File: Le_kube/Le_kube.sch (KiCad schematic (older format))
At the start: 1 part

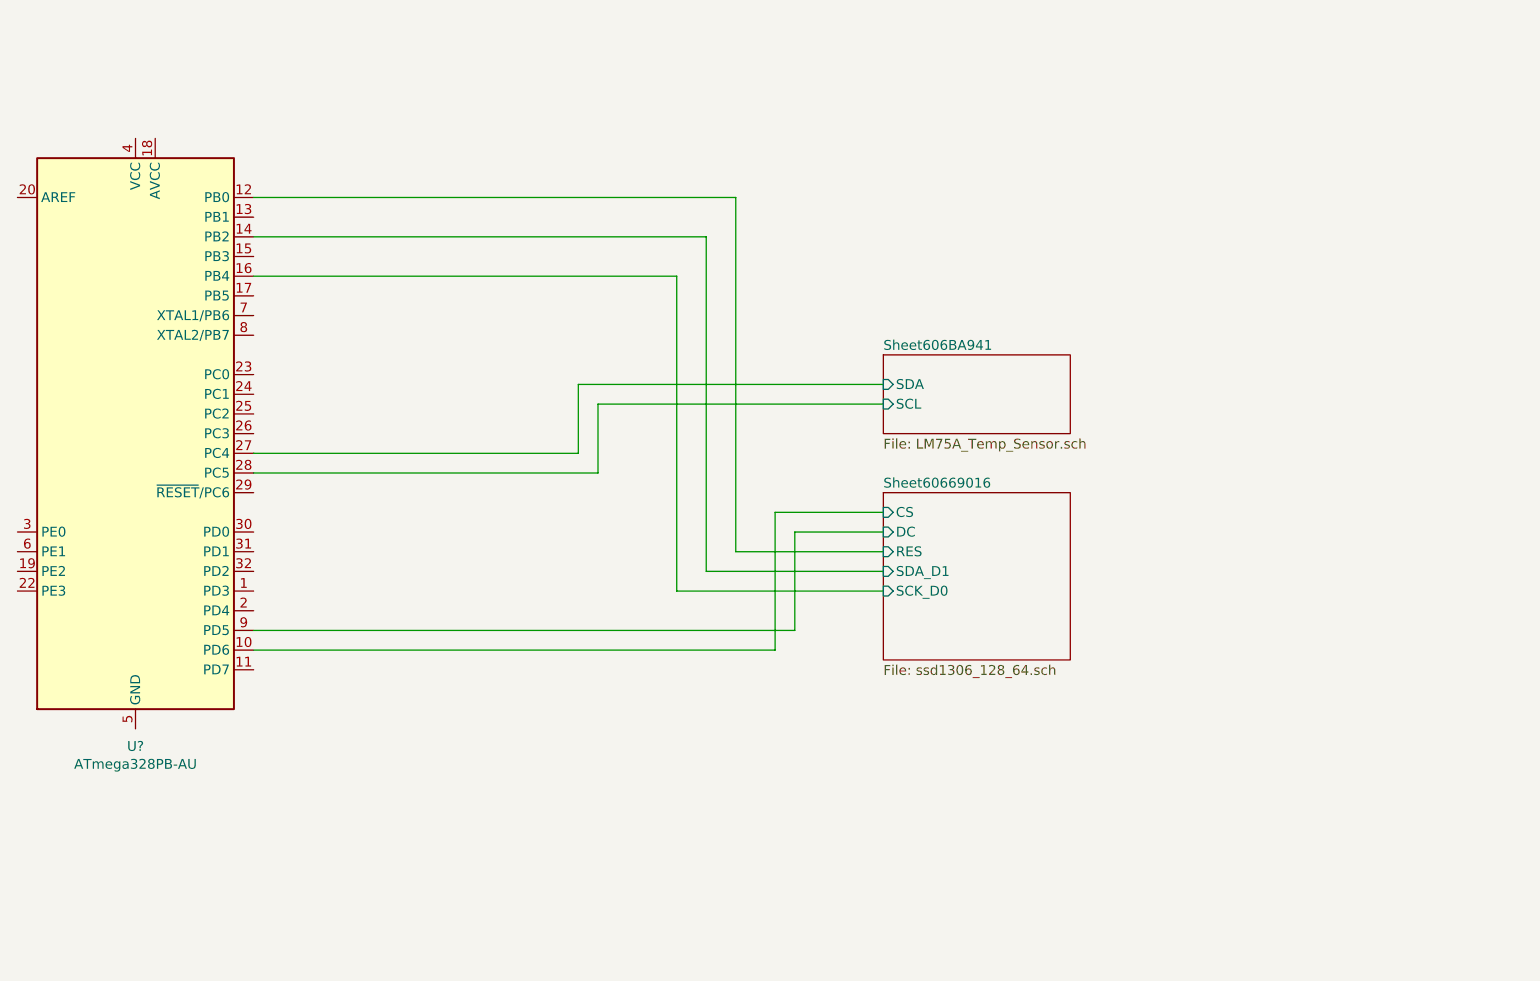
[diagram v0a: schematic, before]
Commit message: cao
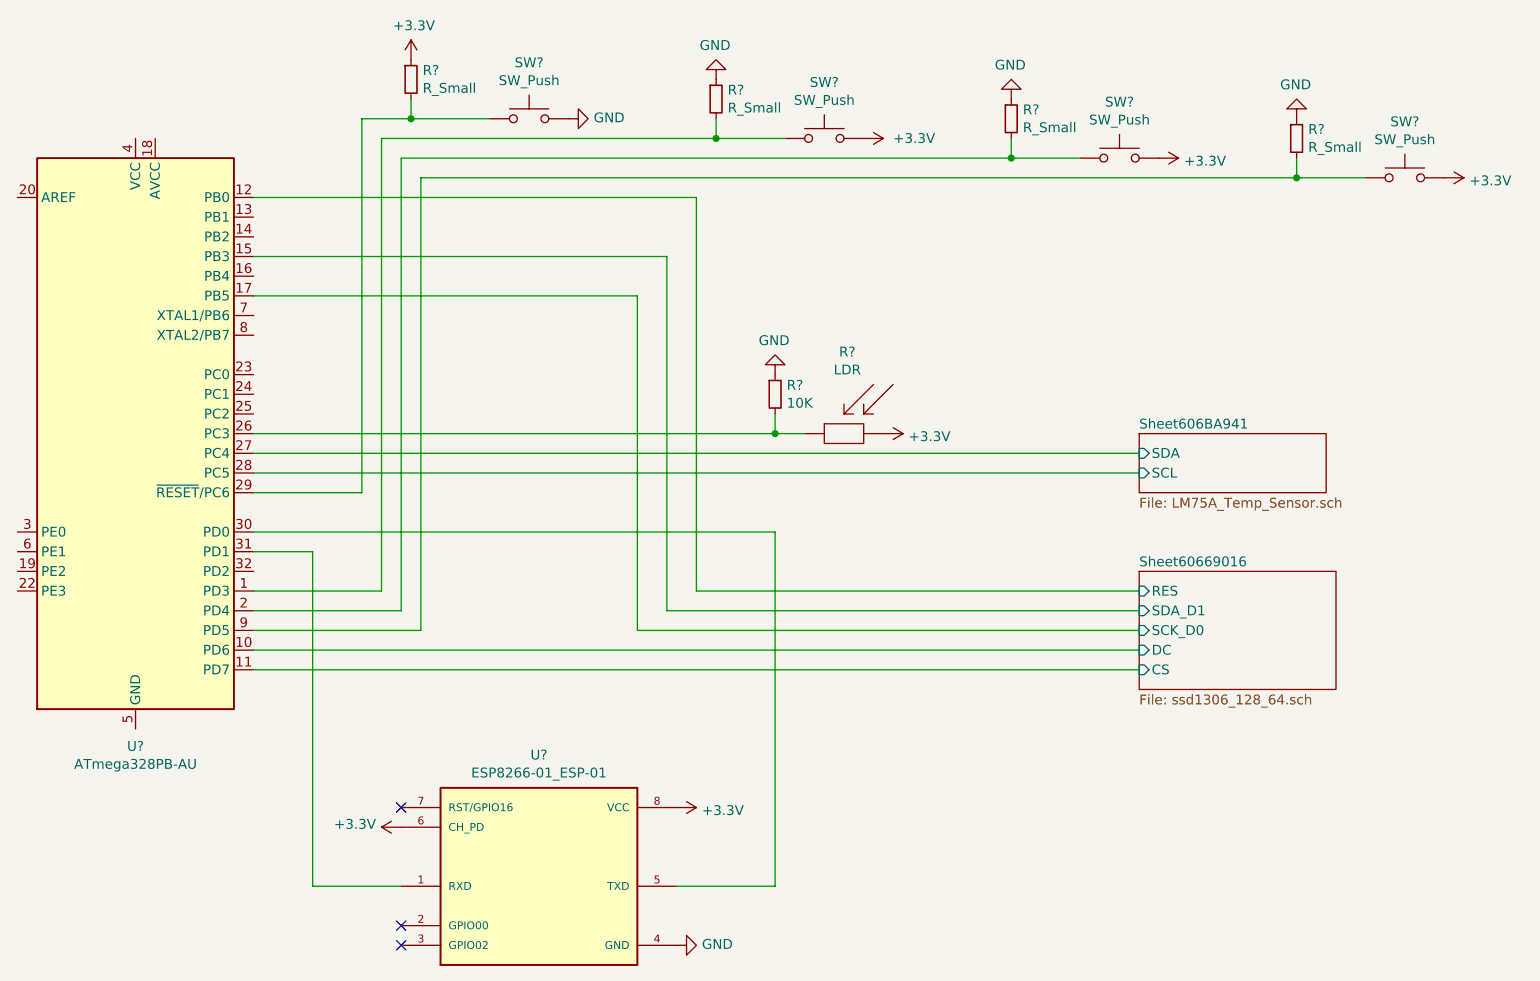
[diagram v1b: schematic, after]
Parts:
- added R?: LDR, symbol Kube_library:LDR
- added R?: 10K, symbol Device:R_Small
- added R? (x4): R_Small, symbol Device:R_Small
- added SW? (x4): SW_Push, symbol Switch:SW_Push
- added U?: ESP8266-01_ESP-01, XCVR_ESP8266-01/ESP-01, symbol ESP01S:ESP8266-01_ESP-01
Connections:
- net Sheet60669016/CS: now also U?.11 (PD7); no longer U?.10 (PD6)
- net Sheet60669016/DC: now also U?.10 (PD6); no longer U?.9 (PD5)
- net Sheet60669016/SCK_D0: now also U?.17 (PB5); no longer U?.16 (PB4)
- net Sheet60669016/SDA_D1: now also U?.15 (PB3); no longer U?.14 (PB2)
- net at U?.1 (PD3): now also R?.2, SW?.1
- net at U?.2 (PD4): now also R?.2, SW?.1
- net at U?.26 (PC3): now also R?.2, R?.~
- net at U?.29 (~RESET~/PC6): now also R?.2, SW?.1
- net at U?.30 (PD0): now also U?.5 (TXD)
- net at U?.31 (PD1): now also U?.1 (RXD)
- new net: R?.2, SW?.1, U?.9 (PD5)
- new net +3V3: R?.1, R?.~, SW?.2, SW?.2, SW?.2, U?.6 (CH_PD), U?.8 (VCC)
- new net GND: R?.1, R?.1, R?.1, R?.1, SW?.2, U?.4 (GND)
- no-connect marks 0 -> 3
